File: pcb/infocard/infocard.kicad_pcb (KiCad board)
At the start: 2 copper layers, 85.6 x 54 mm, 5 parts, among them U1 NT3H2111W0FHKH

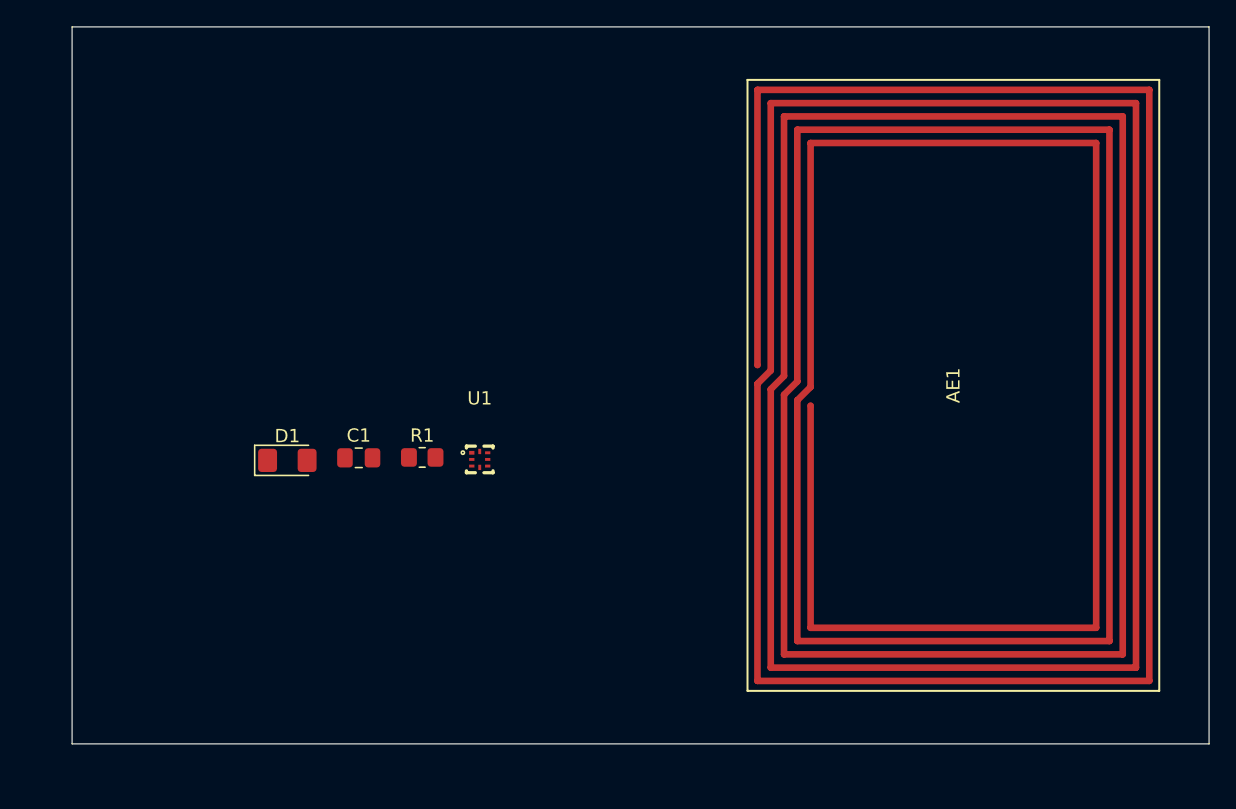
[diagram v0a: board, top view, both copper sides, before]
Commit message: more stuff
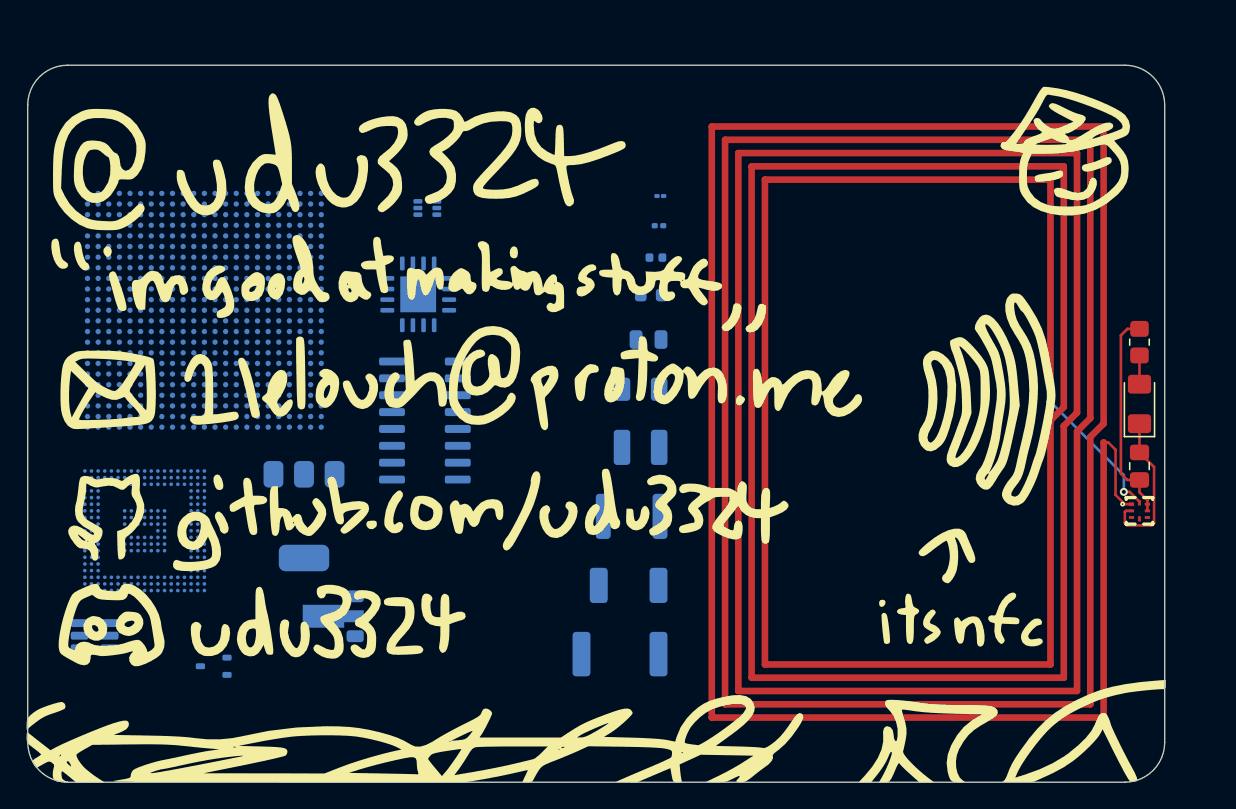
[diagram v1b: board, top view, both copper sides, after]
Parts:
- added G***: LOGO, 1_udu_lib:card_nfc_top, F.Cu at (133.6, 103.8)
- added G***: LOGO, 1_udu_lib:card_nfc_bottom, B.Cu at (132.0, 103.8)
- added REF**: 0201_0603, LED_SMD:LED_0201_0603Metric, B.Cu at (137.5, 87.4)
- added REF**: 2010_5025, LED_SMD:LED_2010_5025Metric, B.Cu at (135.2, 114.5)
- added REF**: SOT-89-3, Package_TO_SOT_SMD:SOT-89-3, B.Cu at (112.7, 116.8)
- added REF**: SOT-223, Package_TO_SOT_SMD:SOT-223, B.Cu at (110.8, 109.3)
- added REF**: 1206_3216, LED_SMD:LED_1206_3216Metric, B.Cu at (136.1, 99.7)
- added REF**: 01005_0402, LED_SMD:LED_01005_0402Metric, B.Cu at (137.6, 85.2)
- added REF**: SOT-23-6, Package_TO_SOT_SMD:SOT-23-6, B.Cu at (95.0, 118.3)
- added REF**: BGA-529_19x19mm_Layout23x23_P0.8mm, Package_BGA:BGA-529_19x19mm_Layout23x23_P0.8mm, B.Cu at (103.3, 93.8)
- added REF**: 0805_2012, LED_SMD:LED_0805_2012Metric, B.Cu at (136.7, 96.0)
- added REF**: SOT-323_SC-70, Package_TO_SOT_SMD:SOT-323_SC-70, B.Cu at (104.0, 120.6)
- added REF**: Xilinx_CPG236, Package_BGA:Xilinx_CPG236, B.Cu at (98.8, 110.4)
- added REF**: 2512_6332, LED_SMD:LED_2512_6332Metric, B.Cu at (134.6, 119.7)
- added REF**: SOIC-16_3.9x9.9mm, Package_SO:SOIC-16_3.9x9.9mm_P1.27mm, B.Cu at (119.9, 102.1)
- added REF**: QFN-16-1EP_5x5mm, Package_DFN_QFN:QFN-16-1EP_5x5mm_P0.8mm_EP2.7x2.7mm, B.Cu at (119.4, 92.6)
- added REF**: 1812_4532, LED_SMD:LED_1812_4532Metric, B.Cu at (135.5, 109.3)
- added REF**: 0603_1608, LED_SMD:LED_0603_1608Metric, B.Cu at (136.9, 92.7)
- added REF**: 0402_1005, LED_SMD:LED_0402_1005Metric, B.Cu at (137.3, 89.8)
- added REF**: SOT-563, Package_TO_SOT_SMD:SOT-563, B.Cu at (120.1, 86.1)
- added REF**: 1210_3225, LED_SMD:LED_1210_3225Metric, B.Cu at (136.1, 104.1)
- moved D1 64.3 mm to (173.7, 100.9), turned to 90 degrees
- moved C1 58.8 mm to (173.7, 105.5), turned to -90 degrees
- moved AE1 58.3 mm to (141.2, 124.7), turned to 90 degrees
- moved R1 54.7 mm to (173.7, 96.2), turned to 90 degrees
- moved U1 49.8 mm to (173.7, 108.9)
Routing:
- net Net-(U1-VCC): track 0.00 -> 16.3 mm
- net Net-(D1-K): track 0.00 -> 11.6 mm
- net Net-(U1-LB): track 0.00 -> 10.7 mm, vias 0 -> 2
- net Net-(U1-LA): track 0.00 -> 6.02 mm
- net Net-(D1-A): track 0.00 -> 2.26 mm
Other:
- outline, holes or cut-outs redrawn
- board text added: "Imperial - Metric"
